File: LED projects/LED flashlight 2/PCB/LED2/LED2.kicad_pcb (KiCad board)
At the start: 2 copper layers, 21 x 12.5 mm, 5 parts, among them SW1 SW_Push

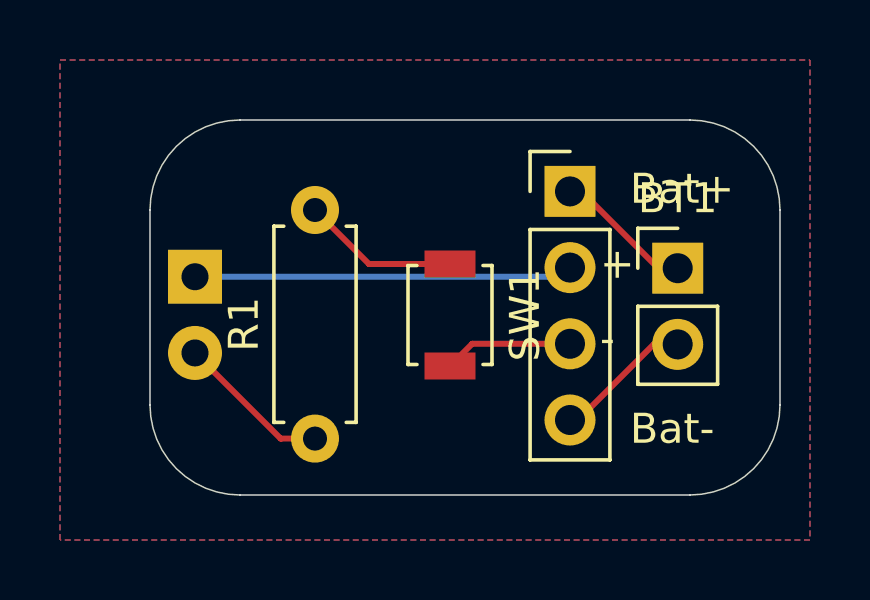
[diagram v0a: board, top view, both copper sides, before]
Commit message: update
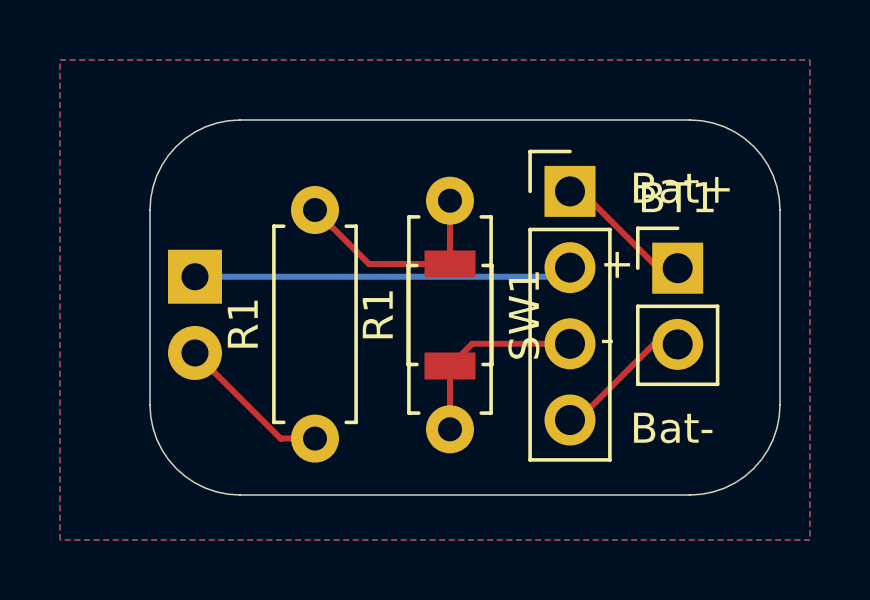
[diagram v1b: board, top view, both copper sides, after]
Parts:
- added R1: R_US, Resistor_THT:R_Axial_DIN0207_L6.3mm_D2.5mm_P7.62mm_Horizontal, F.Cu at (152.1, 103.1)
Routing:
- net Net-(R1-Pad2): track 5.25 -> 7.36 mm
- net Net-(BatteryChargeModule1--): track 4.31 -> 6.42 mm
